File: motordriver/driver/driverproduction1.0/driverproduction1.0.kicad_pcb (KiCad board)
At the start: 4 copper layers, 28 parts

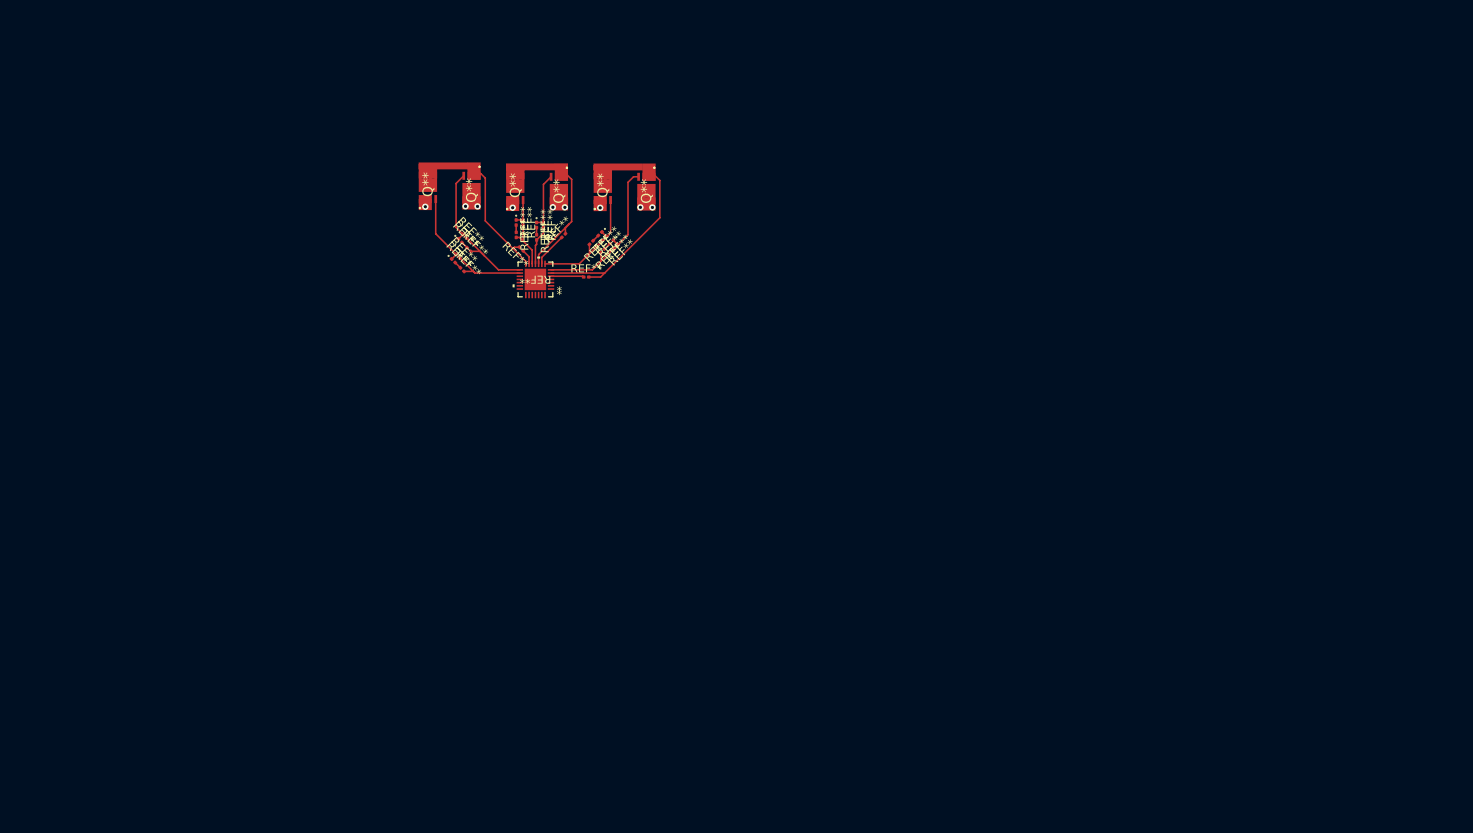
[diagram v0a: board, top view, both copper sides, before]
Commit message: l
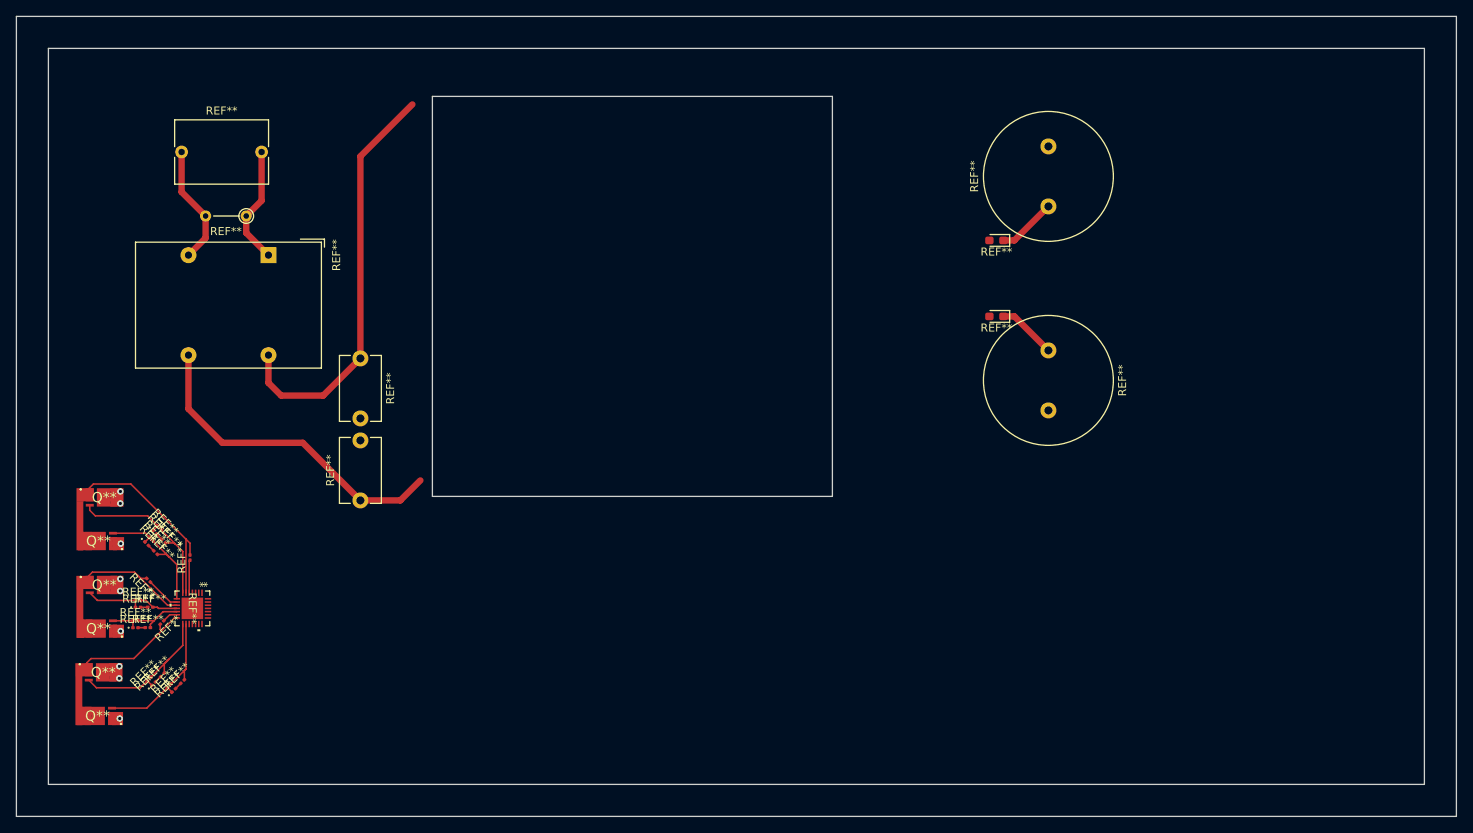
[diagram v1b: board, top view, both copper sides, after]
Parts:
- added REF**: R_Axial_DIN0204_L3.6mm_D1.6mm_P5.08mm_Vertical, Resistor_THT:R_Axial_DIN0204_L3.6mm_D1.6mm_P5.08mm_Vertical, F.Cu at (58.7, 45.0)
- added REF**: C_Disc_D8.0mm_W5.0mm_P7.50mm, Capacitor_THT:C_Disc_D8.0mm_W5.0mm_P7.50mm, F.Cu at (73.0, 62.8)
- added REF**: C_Rect_L11.5mm_W7.8mm_P10.00mm_MKT, Capacitor_THT:C_Rect_L11.5mm_W7.8mm_P10.00mm_MKT, F.Cu at (50.6, 37.0)
- added REF**: Choke_Schaffner_RN216-04-15.5x23.0mm, Inductor_THT:Choke_Schaffner_RN216-04-15.5x23.0mm, F.Cu at (61.5, 49.8)
- added REF**: C_Radial_D16.0mm_H25.0mm_P7.50mm, Capacitor_THT:C_Radial_D16.0mm_H25.0mm_P7.50mm, F.Cu at (159.0, 43.8)
- added REF**: D_0603_1608Metric_Pad1.05x0.95mm_HandSolder, Diode_SMD:D_0603_1608Metric_Pad1.05x0.95mm_HandSolder, F.Cu at (152.5, 48.0)
- added REF**: C_Disc_D8.0mm_W5.0mm_P7.50mm, Capacitor_THT:C_Disc_D8.0mm_W5.0mm_P7.50mm, F.Cu at (73.0, 80.5)
- added REF**: D_0603_1608Metric_Pad1.05x0.95mm_HandSolder, Diode_SMD:D_0603_1608Metric_Pad1.05x0.95mm_HandSolder, F.Cu at (152.5, 57.5)
- added REF**: C_Radial_D16.0mm_H25.0mm_P7.50mm, Capacitor_THT:C_Radial_D16.0mm_H25.0mm_P7.50mm, F.Cu at (159.0, 61.8)
- moved Q** 78.4 mm to (40.6, 80.1), turned to 180 degrees
- moved Q** 77.7 mm to (40.5, 107.4), turned to 0 degrees
- moved Q** 76.6 mm to (40.6, 85.6), turned to 0 degrees
- moved Q** 76.4 mm to (40.5, 102.0), turned to 180 degrees
- moved Q** 75.7 mm to (40.6, 91.1), turned to 180 degrees
- moved Q** 75.5 mm to (40.6, 96.5), turned to 0 degrees
- moved REF** 69.5 mm to (44.9, 96.4), turned to 0 degrees
- moved REF** 69.5 mm to (44.9, 95.5), turned to 0 degrees
- moved REF** 69.1 mm to (45.2, 93.0), turned to 0 degrees
- moved REF** 69.0 mm to (45.2, 93.9), turned to 0 degrees
- moved REF** 68.7 mm to (46.3, 85.9), turned to -45 degrees
- moved REF** 68.0 mm to (46.9, 85.3), turned to -45 degrees
- moved REF** 68.0 mm to (46.6, 102.8), turned to 45 degrees
- moved REF** 67.6 mm to (47.3, 84.5), turned to -45 degrees
- moved REF** 67.4 mm to (46.5, 90.5), turned to 135 degrees
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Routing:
- net (no net): track 251.1 -> 420.2 mm
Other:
- board outline added: 180 x 100 mm
